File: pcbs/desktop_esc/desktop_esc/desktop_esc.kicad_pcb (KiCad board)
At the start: 2 copper layers, 100 x 75 mm, 36 parts, among them J1 Conn_02x10_Odd_Even, J2 Conn_01x12_Female, J3 Conn_01x03_Female, J7 Conn_01x02_Female, U1 Pico, U2 AP1117-33, U3 ajm_cd40109, U4 ajm_cd40109, U5 ajm_cd40109, U6 ajm_cd40109

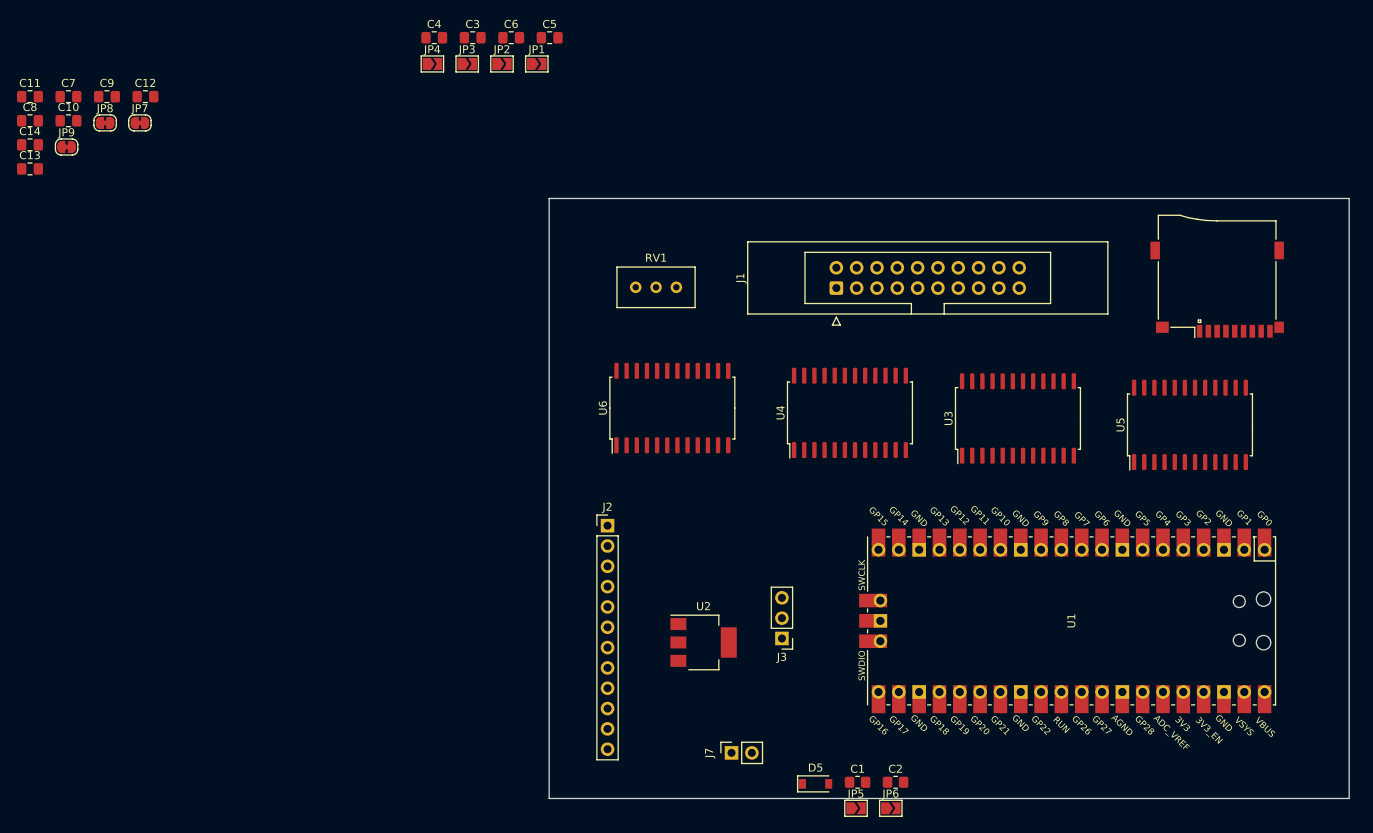
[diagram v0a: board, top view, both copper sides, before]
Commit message: Updates
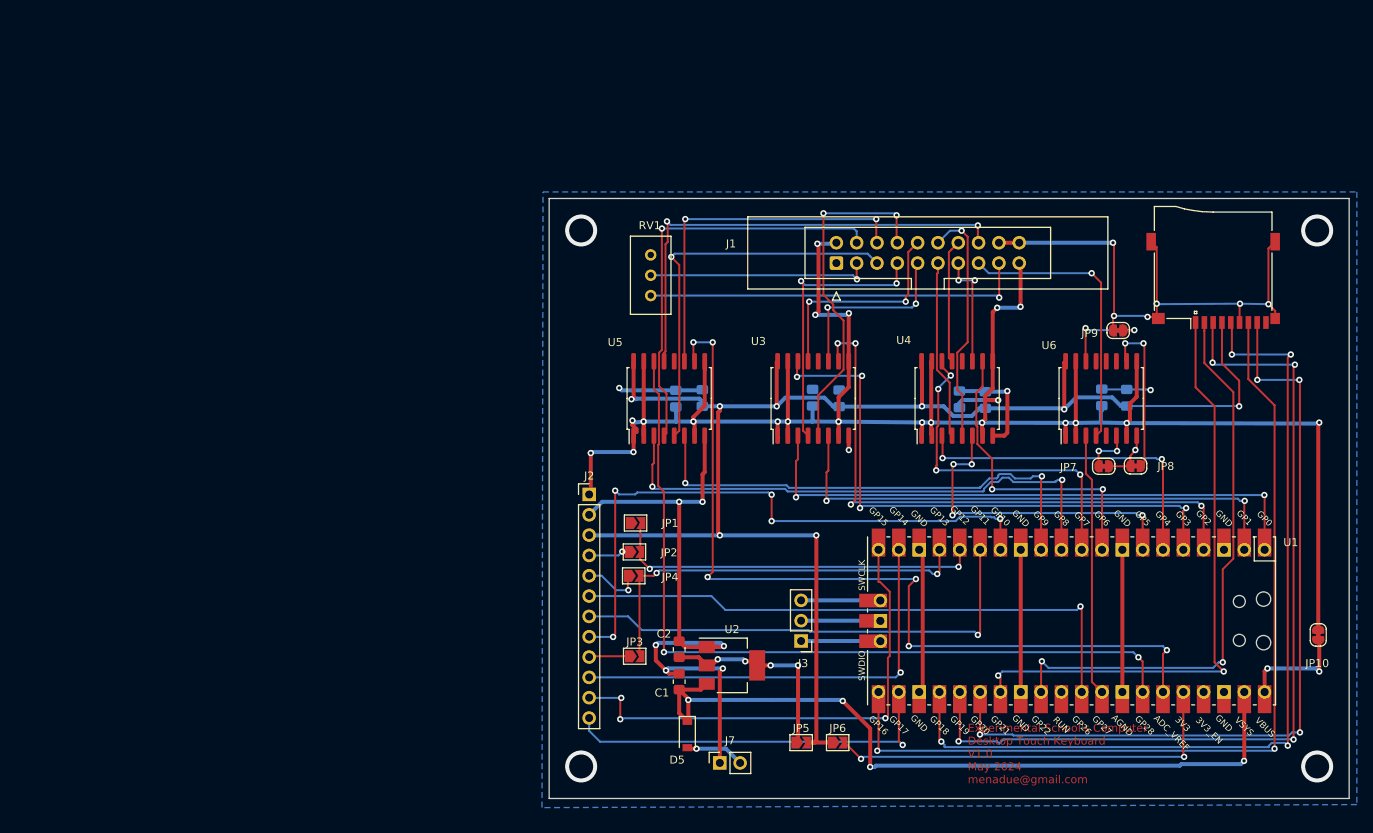
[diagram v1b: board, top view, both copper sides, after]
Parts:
- removed C3, C4, C5, C6: C_Small, Capacitor_SMD:C_0805_2012Metric_Pad1.18x1.45mm_HandSolder
- added JP10: Jumper_NC_Small, Jumper:SolderJumper-2_P1.3mm_Bridged_RoundedPad1.0x1.5mm, F.Cu at (191.1, 114.6)
- C10, C11, C12, C13, C14, C7, C8, C9: moved to B.Cu
- U3, U4, U5, U6: footprint Package_SO:SOP-24_7.5x15.4mm_P1.27mm -> Package_SO:SOIC-16W_7.5x10.3mm_P1.27mm
- moved C13 140.0 mm to (167.2, 84.9), turned to 90 degrees
- moved C14 137.6 mm to (164.1, 84.9), turned to 90 degrees
- moved JP8 135.8 mm to (168.3, 93.4), turned to 180 degrees
- moved JP9 133.4 mm to (166.1, 76.5), turned to 180 degrees
- moved JP7 127.9 mm to (164.3, 93.5)
- moved C10 116.7 mm to (146.3, 85.1), turned to 90 degrees
- moved C9 116.2 mm to (149.5, 85.2), turned to 90 degrees
- moved C8 103.8 mm to (127.9, 84.9), turned to 90 degrees
- moved C7 103.4 mm to (131.2, 85.0), turned to 90 degrees
- moved C11 92.1 mm to (114.1, 84.9), turned to 90 degrees
- moved JP3 76.9 mm to (105.7, 117.2)
- moved C12 76.3 mm to (110.8, 85.0), turned to 90 degrees
- moved JP4 68.8 mm to (105.6, 107.2)
- moved U5 65.2 mm to (110.0, 85.0)
- moved JP2 63.2 mm to (105.7, 104.2)
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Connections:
- J2 pad 11: (no net) -> DBG_CLK_3V3
- J2 pad 12: (no net) -> WS_3V3
- U1 pad 20: DBG_CLK_3V4 -> DBG_CLK_3V3
- U1 pad 22: WS_3V5 -> WS_3V3
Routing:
- net +5V: track 0.00 -> 261.2 mm, vias 0 -> 21
- net GND: track 0.00 -> 240.0 mm, vias 0 -> 17
- net +3V3: track 0.00 -> 187.2 mm, vias 0 -> 8
- net MISO_D0: track 0.00 -> 111.8 mm, vias 0 -> 2
- net SD_CLK: track 0.00 -> 111.0 mm, vias 0 -> 4
- net MOSI_DI: track 0.00 -> 110.8 mm, vias 0 -> 4
- net A0_3V3: track 0.00 -> 107.2 mm, vias 0 -> 6
- net SD_DAT1: track 0.00 -> 102.1 mm, vias 0 -> 4
- net RESET_N_3V3: track 0.00 -> 101.1 mm, vias 0 -> 2
- net VSYS: track 0.00 -> 97.3 mm, vias 0 -> 4
- net SCK_3V3: track 0.00 -> 77.5 mm, vias 0 -> 5
- net SD_DAT2: track 0.00 -> 75.7 mm, vias 0 -> 2
- net DB2_3V3: track 0.00 -> 74.6 mm, vias 0 -> 4
- net DB0_3V3: track 0.00 -> 73.3 mm, vias 0 -> 2
- net DB3_3V3: track 0.00 -> 73.2 mm, vias 0 -> 4
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- added copper zone on B.Cu, net GND
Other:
- board text added: "Experimental School's Computer Desktop Touch Keyboard V1.0 May 2024 menadue@gmail.com"
